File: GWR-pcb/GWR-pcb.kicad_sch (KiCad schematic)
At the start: 47 parts, among them J1 Conn_01x11, J2 Conn_01x12, M1 Motor_DC, Q1 AO3400A, SW1 SW_DIP_x01, SW2 Angled_Mode, SW3 Angled_RST, U1 AMS1117-1.5, U2 XIAO-ESP32-S3-Plus-SMD, U3 MAX98357A, U4 74AUP1G32, U5 MCP23S17x-x-SS, U6 ADXL343

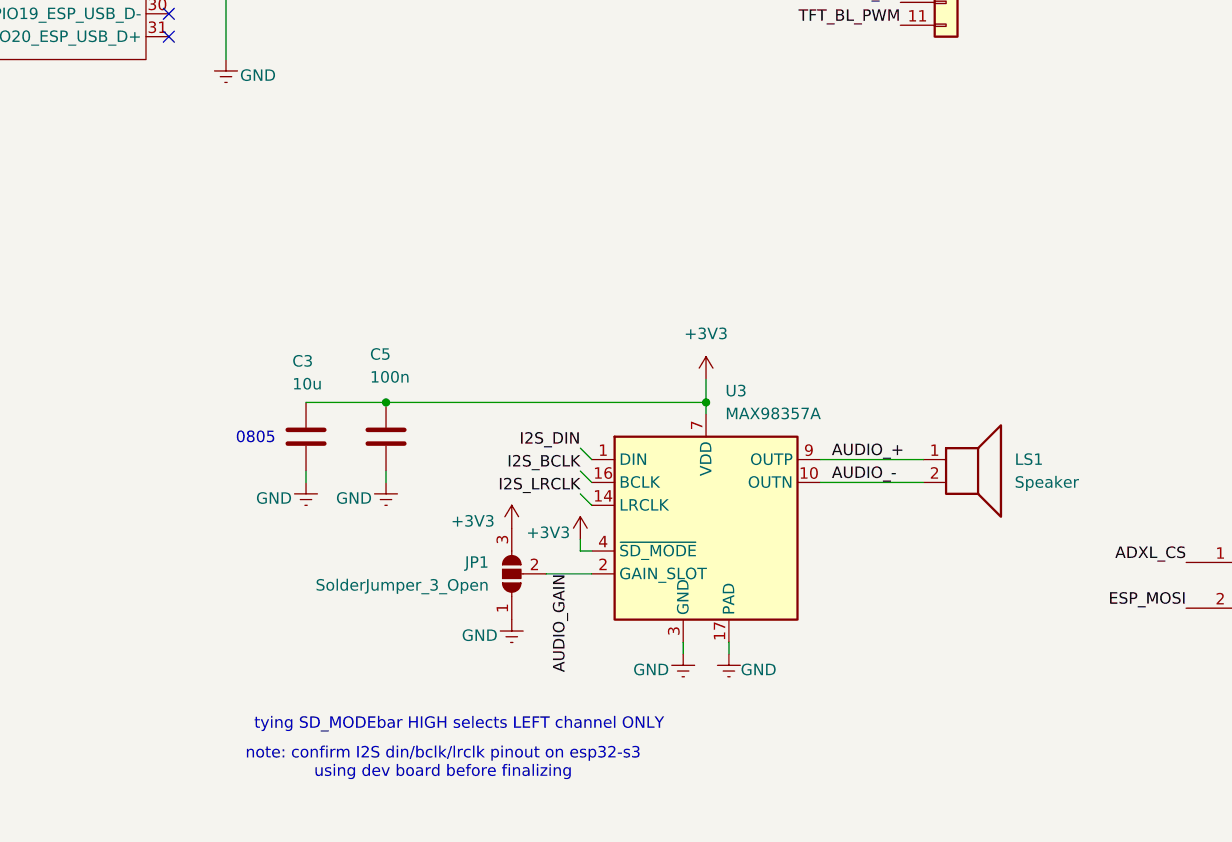
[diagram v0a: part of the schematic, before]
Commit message: pcb layout changes
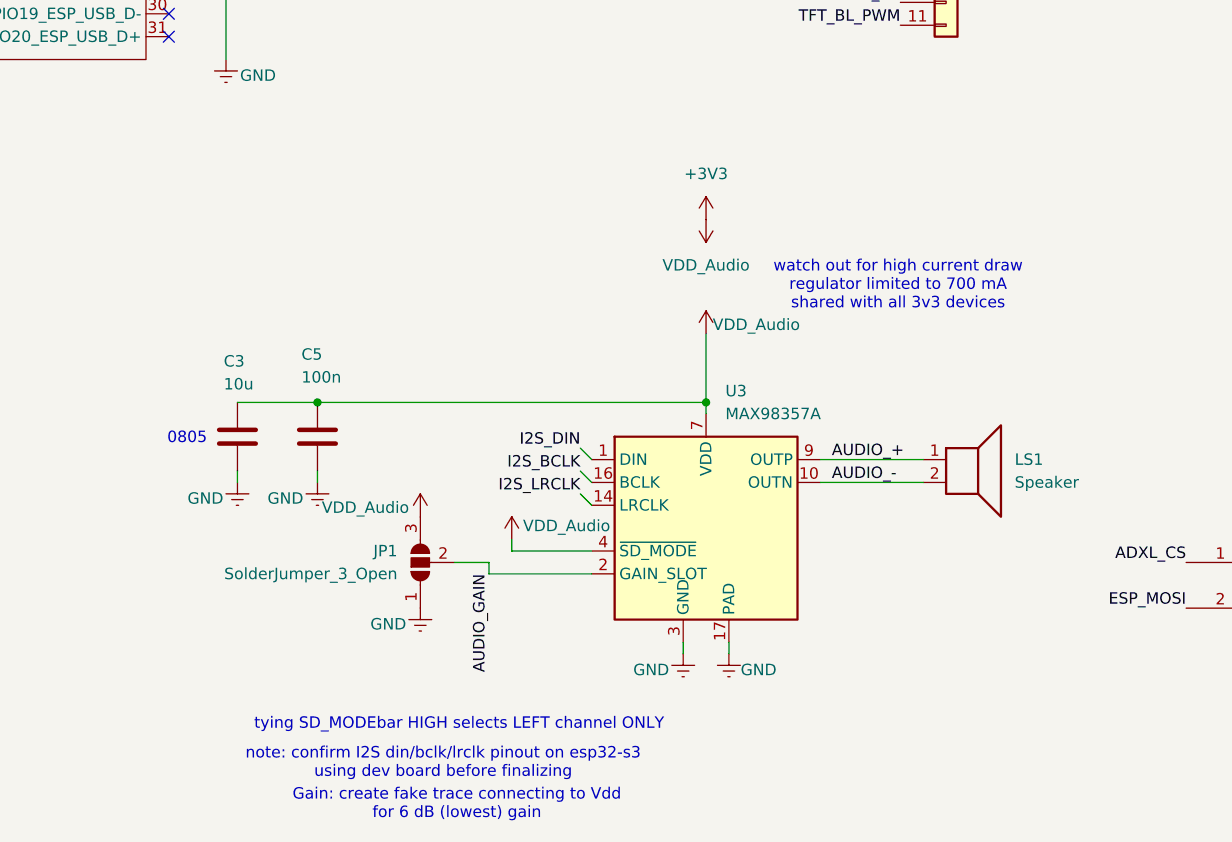
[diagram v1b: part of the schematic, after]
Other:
- note added: "Gain: create fake trace connecting to Vdd for 6 dB (lowest) gain"
- note added: "watch out for high current draw regulator limited to 700 mA shared with all 3v3 devices"
- moved on the sheet: C3, C5, JP1
